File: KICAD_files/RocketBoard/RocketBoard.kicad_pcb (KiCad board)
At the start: 2 copper layers, 49.2 x 117.6 mm, 23 parts, among them J1 GY-BME-280 Barometer, J5 Buzzer, K1 SRD-05VDC-SL-C, Q1 2N2222, SW1 RESET, SW2 ON/OFF, U1 RPI-Pico, U2 L7805, U3 ESP32-CAM

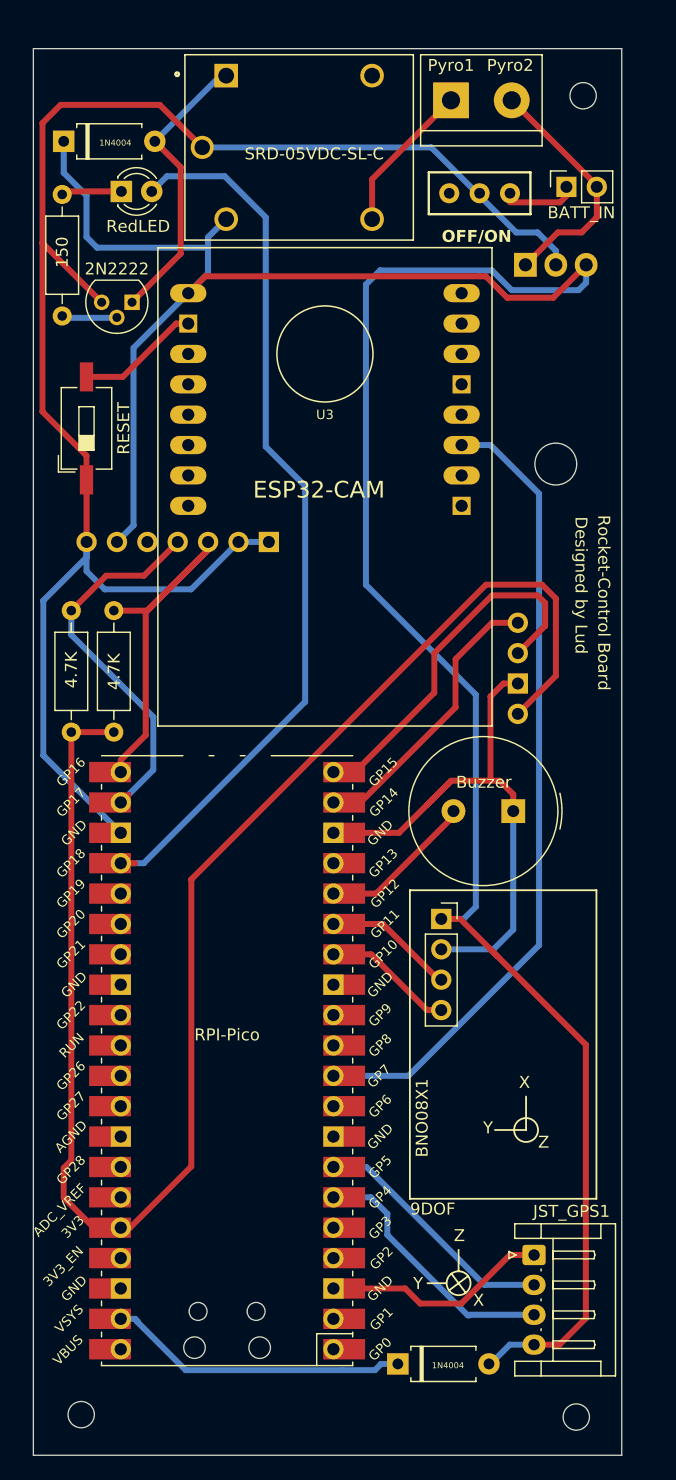
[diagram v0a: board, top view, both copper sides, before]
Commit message: hhbh
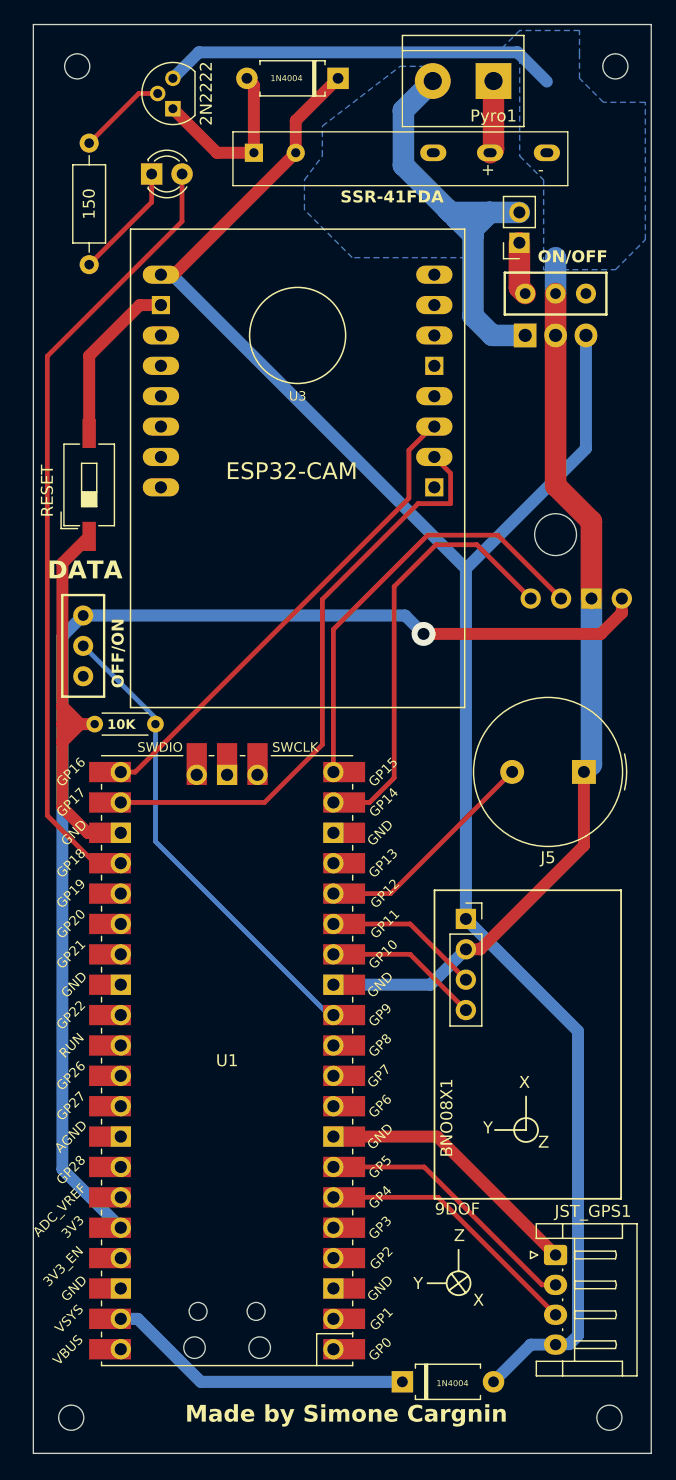
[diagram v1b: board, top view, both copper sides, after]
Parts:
- removed LORA_Socket1: LORA_Socket, Connector_PinSocket_2.54mm:PinSocket_1x07_P2.54mm_Vertical
- removed R2: 4.7K, Resistor_THT:R_Axial_DIN0207_L6.3mm_D2.5mm_P10.16mm_Horizontal
- removed REF** (x3): MountingHole_2.2mm_M2, MountingHole:MountingHole_2.2mm_M2
- added H1: MountingHole, MountingHole:MountingHole_2.1mm, F.Cu at (146.5, 148.0)
- added H2: MountingHole, MountingHole:MountingHole_2.1mm, F.Cu at (147.0, 35.0)
- added H3: MountingHole, MountingHole:MountingHole_2.1mm, F.Cu at (102.0, 35.0)
- added H4: MountingHole, MountingHole:MountingHole_2.1mm, F.Cu at (101.5, 148.0)
- added SW3: ON/OFF, roba_mia:Schiebeschalter SS-12D00, F.Cu at (102.5, 83.5)
- BATT1: renamed from BATT_IN1; value BATT_IN -> ~
- J5: value Buzzer -> PassiveBuzzer; footprint Buzzer_Beeper:Buzzer_TDK_PS1240P02BT_D12.2mm_H6.5mm -> roba_mia:myBuzzer
- K1: footprint Relay5V:RELAY_SRD-05VDC-SL-C -> roba_mia:ssr-41FDA
- Pyro1: value Pyro2 -> ~
- R1: value 4.7K -> 10K omh; footprint Resistor_THT:R_Axial_DIN0207_L6.3mm_D2.5mm_P10.16mm_Horizontal -> Resistor_THT:R_Axial_DIN0204_L3.6mm_D1.6mm_P5.08mm_Horizontal
- U1: footprint MCU_RaspberryPi_and_Boards:RPi_Pico_SMD_TH_2 -> raspberry pi pico:RPi_Pico_SMD_TH
- moved D3 23.5 mm to (123.8, 36.0), turned to 180 degrees
- moved Q1 16.5 mm to (110.0, 38.5), turned to 90 degrees
- moved J1 13.0 mm to (147.5, 79.5), turned to 90 degrees
- moved SW2 10.5 mm to (142.0, 54.0), turned to 0 degrees
- moved J5 6.32 mm to (143.8, 94.0)
- moved R3 6.29 mm to (103.0, 51.6), turned to 90 degrees
- moved BATT1 6.11 mm to (138.9, 49.8), turned to 180 degrees
- moved K1 5.99 mm to (125.7, 44.7)
- moved U2 5.90 mm to (139.4, 57.5)
- moved SW1 4.74 mm to (103.0, 70.0)
- moved Pyro1 3.91 mm to (136.8, 36.2), turned to 180 degrees
- moved D2 2.92 mm to (108.2, 44.0)
- moved U3 2.76 mm to (120.4, 62.6)
- moved BNO08X1 2.06 mm to (134.5, 106.3)
- moved JST_GPS1 1.80 mm to (142.0, 134.4)
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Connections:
- net Net-(BATT_IN1-Pin_1) renamed /battGNDpreSwitch
- net Net-(D1-K) renamed /5V 
- net Net-(D3-A) renamed /Relè_GND_signal
- net Net-(U3-GND@3) renamed /esp32_GND
- net WIRE renamed /batt_vcc
- K1 pad COM: GND -> /batt_GND_after_relè
- K1 pad NO: Net-(Pyro1-Pin_1) -> GND
- Pyro1 pad 1: Net-(Pyro1-Pin_1) -> /batt_GND_after_relè
- R1 pad 1: +3.3V -> GND
- R1 pad 2: Net-(LORA_Socket1-Pin_3) -> Net-(SW3-B)
- U1 pad 10: Net-(U1-GPIO7) -> unconnected-(U1-GPIO7-Pad10)
- U1 pad 12: unconnected-(U1-GPIO9-Pad12) -> Net-(SW3-B)
- U1 pad 21: Net-(LORA_Socket1-Pin_3) -> Net-(U1-GPIO16)
- U1 pad 22: Net-(LORA_Socket1-Pin_4) -> Net-(U1-GPIO17)
- U1 pad 28: GND -> unconnected-(U1-GND-Pad28)
- U1 pad 30: unconnected-(U1-RUN-Pad30) -> GND
- U1 pad 8: unconnected-(U1-GND-Pad8) -> GND
- U3 pad P$2: unconnected-(U3-GPIO1-PadP$2) -> Net-(U1-GPIO17)
- U3 pad P$3: Net-(U1-GPIO7) -> Net-(U1-GPIO16)
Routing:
- net Net-(U1-GPIO7): track 67.6 -> 0.00 mm
- net +5V: track 216.7 -> 158.6 mm
- net Net-(U1-GPIO17): track 0.00 -> 49.5 mm
- net Net-(U1-GPIO16): track 0.00 -> 40.5 mm
- net GND: track 209.0 -> 168.8 mm
- net Net-(SW3-B): track 0.00 -> 39.7 mm
- net Net-(LORA_Socket1-Pin_3): track 32.3 -> 0.00 mm
- net Net-(LORA_Socket1-Pin_4): track 31.7 -> 0.00 mm
- net +3.3V: track 132.7 -> 101.5 mm, vias 0 -> 1
- net /batt_vcc: track 20.3 -> 36.7 mm
- net Net-(Pyro1-Pin_1): track 12.7 -> 0.00 mm
- net Net-(J1-Pin_4): track 24.0 -> 36.7 mm
- net /Relè_GND_signal: track 25.0 -> 14.8 mm
- net Net-(D2-A): track 75.6 -> 66.1 mm
- net /batt_GND_after_relè: track 0.00 -> 6.53 mm
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- added copper zone on B.Cu, net /batt_vcc
- added copper zone on B.Cu, net GND
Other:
- board size 49.2 x 117.6 mm -> 51.7 x 119.5 mm
- board text added: "10K"
- board text added: "DATA"
- board text added: "Made by Simone Cargnin"
- board text added: "ON/OFF"
- board text added: "SSR-41FDA"
- board text removed: "4.7K"
- board text removed: "Designed by Lud"
- board text removed: "Made in collaboration with Simone Cargnin & Vittorio Sedda"
- board text removed: "Rocket-Control Board"
- board text removed: "Sbirro guarda un po' più in la del tuo binocolo Non c'è una scelta se i bisogni te li impongono"
